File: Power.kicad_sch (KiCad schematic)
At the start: 26 parts, among them SW1 SHPHLD, U3 NPM1304-QEAA-R

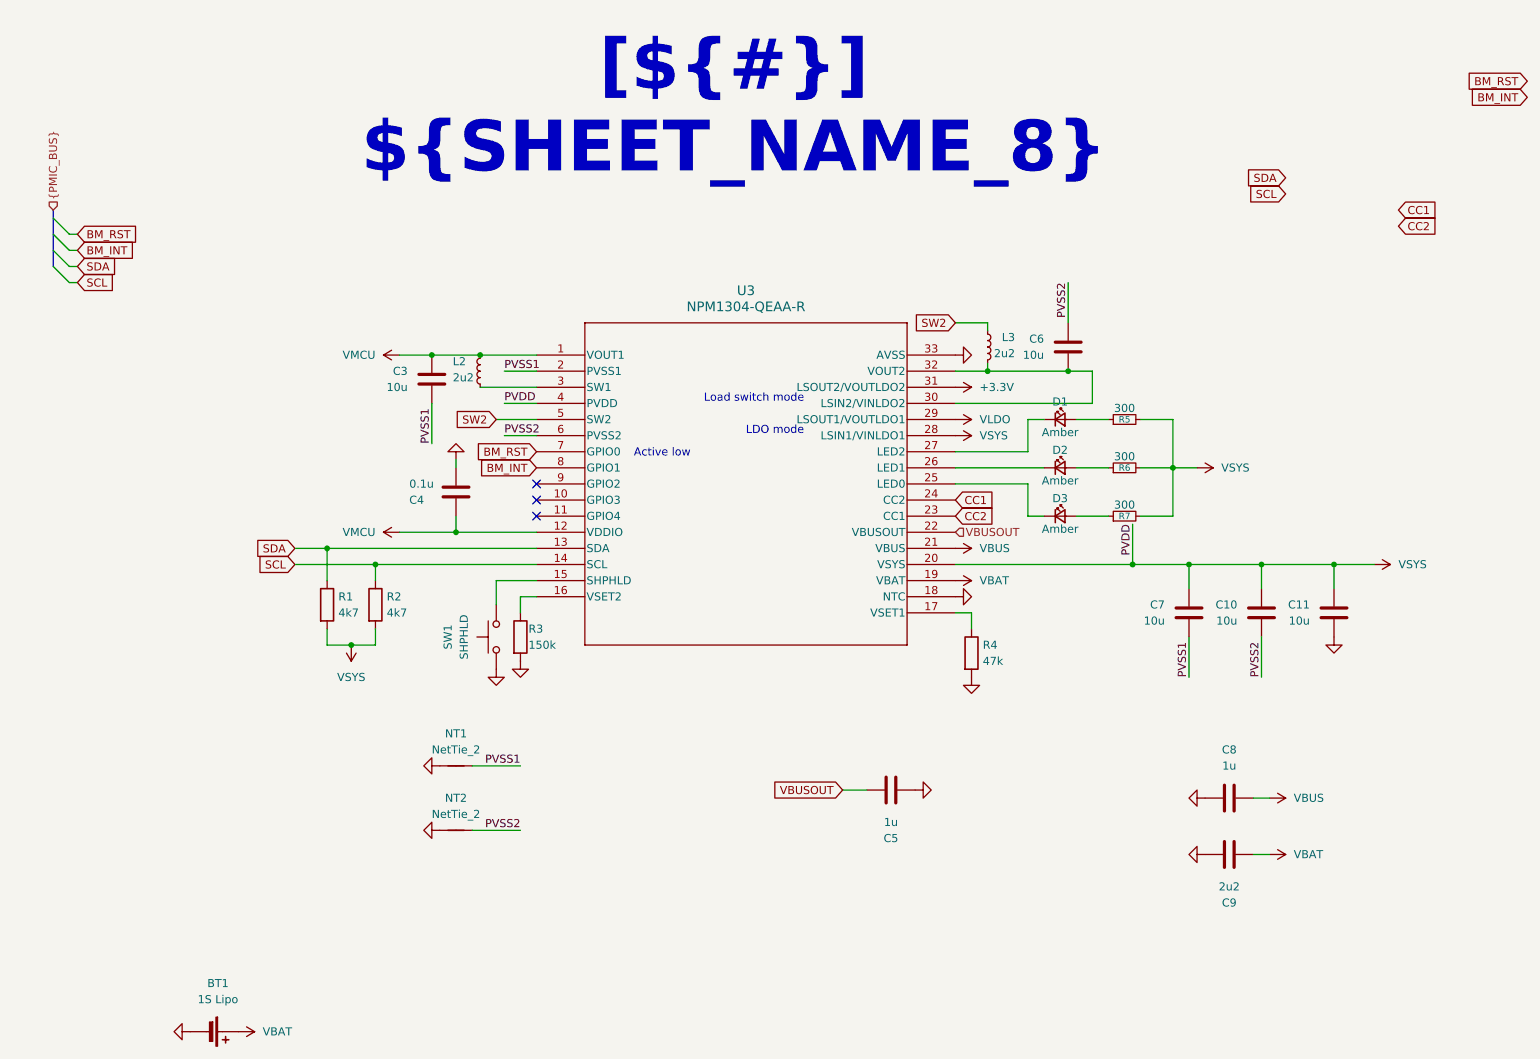
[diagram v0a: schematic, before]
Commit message: Edited ci.yaml
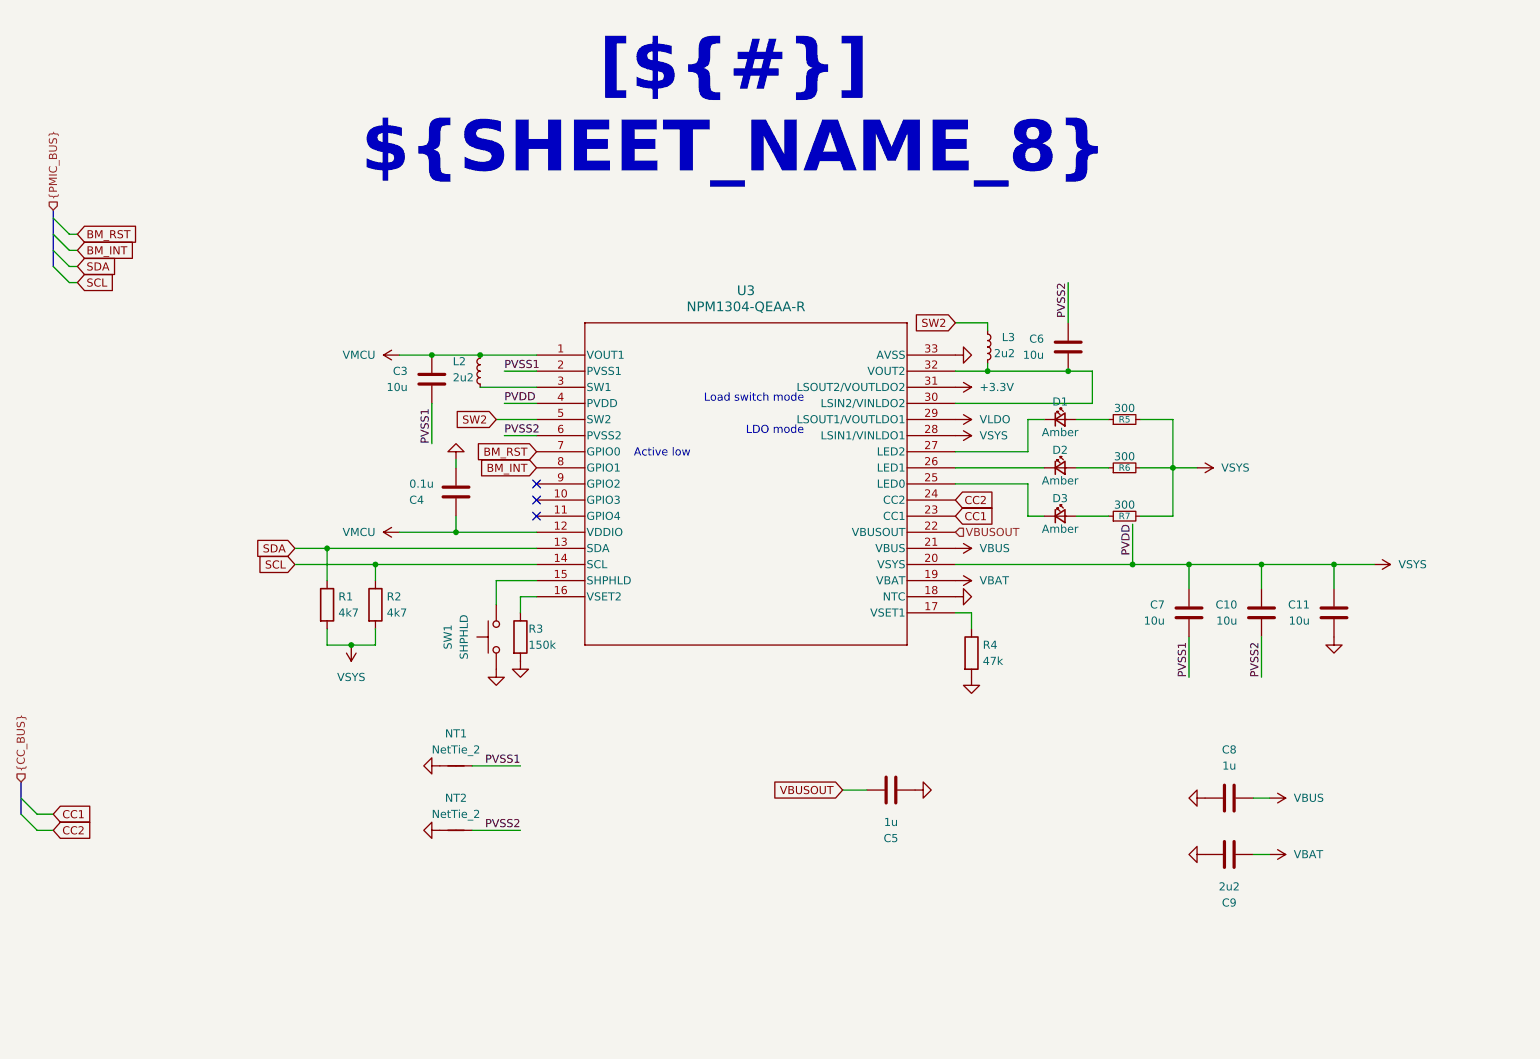
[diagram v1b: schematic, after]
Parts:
- removed BT1: 1S Lipo, Connector_JST:JST_XH_B2B-XH-A_1x02_P2.50mm_Vertical, symbol Device:Battery_Cell
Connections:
- net CC1: now also U3.23 (CC1); no longer U3.24 (CC2)
- net CC2: now also U3.24 (CC2); no longer U3.23 (CC1)
